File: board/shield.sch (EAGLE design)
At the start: 45 parts, among them IC1 LM75, J1 22-05-7048-04, J2 22-05-7028-02, J4 POWER_JACKPTH, K1 G5L, T1 BC817, U1 LM2596S-5.0

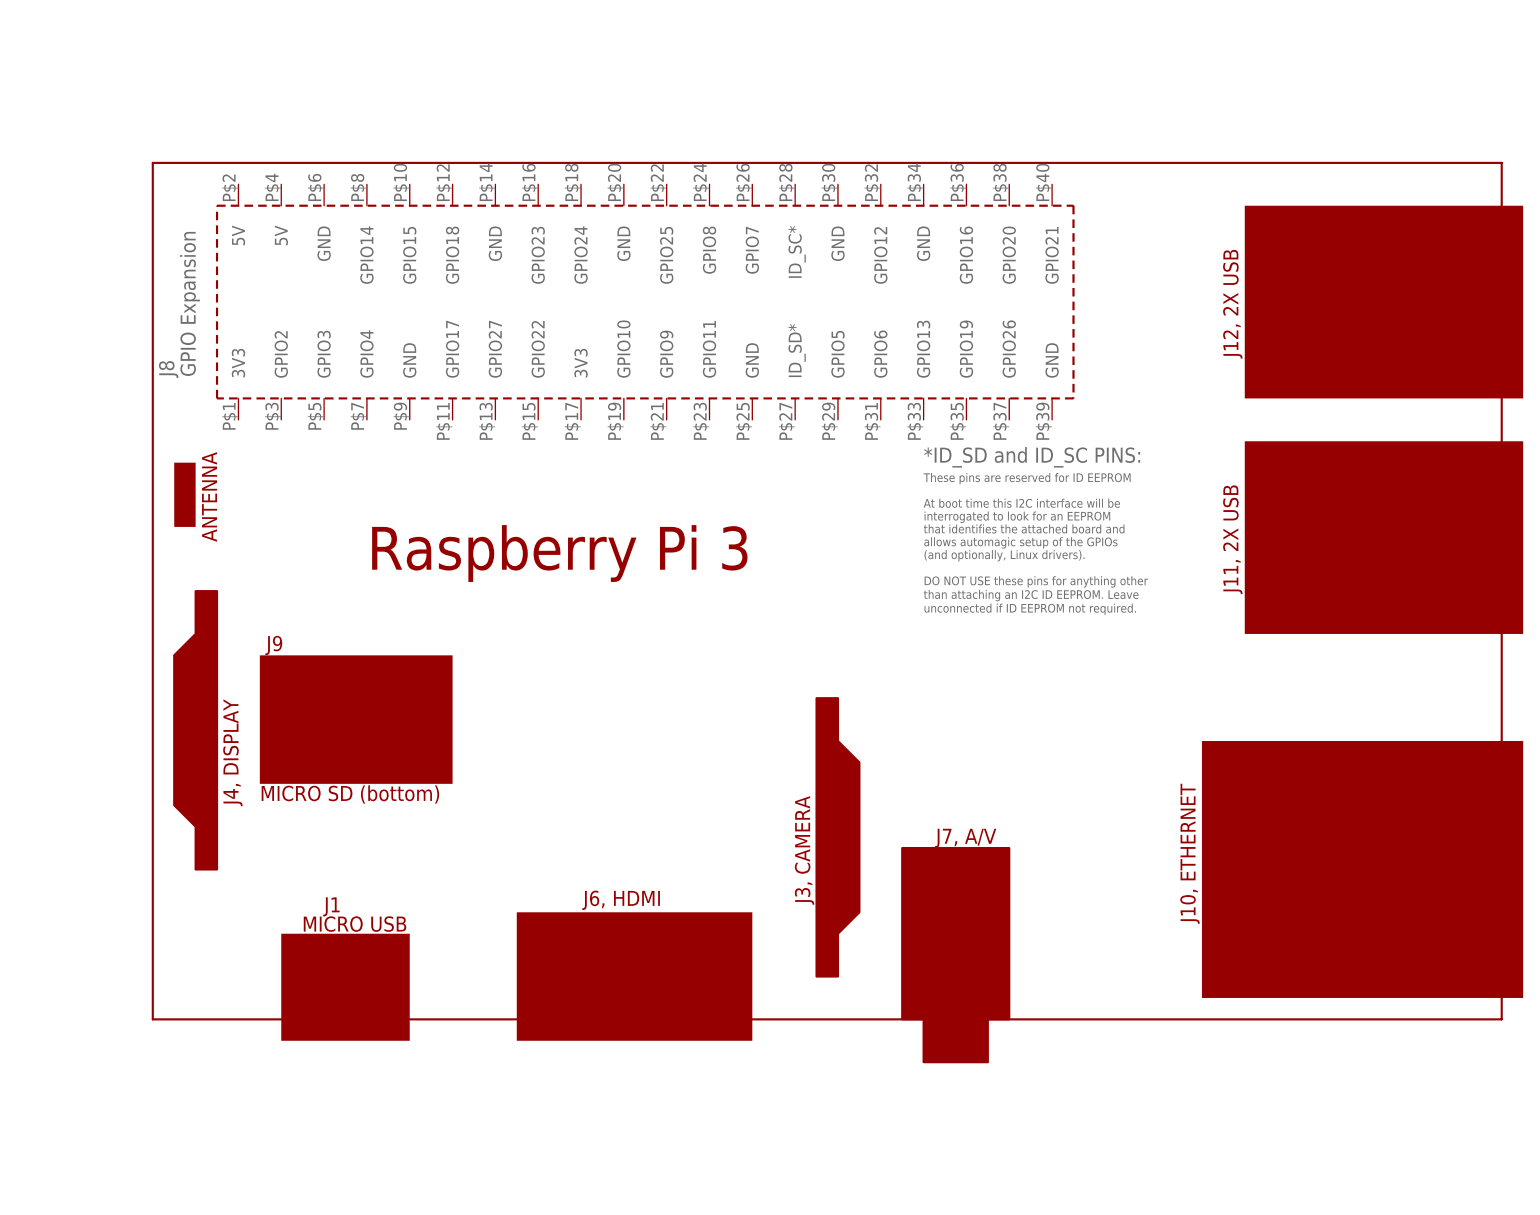
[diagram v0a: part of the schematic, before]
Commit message: Silkscreen corrected
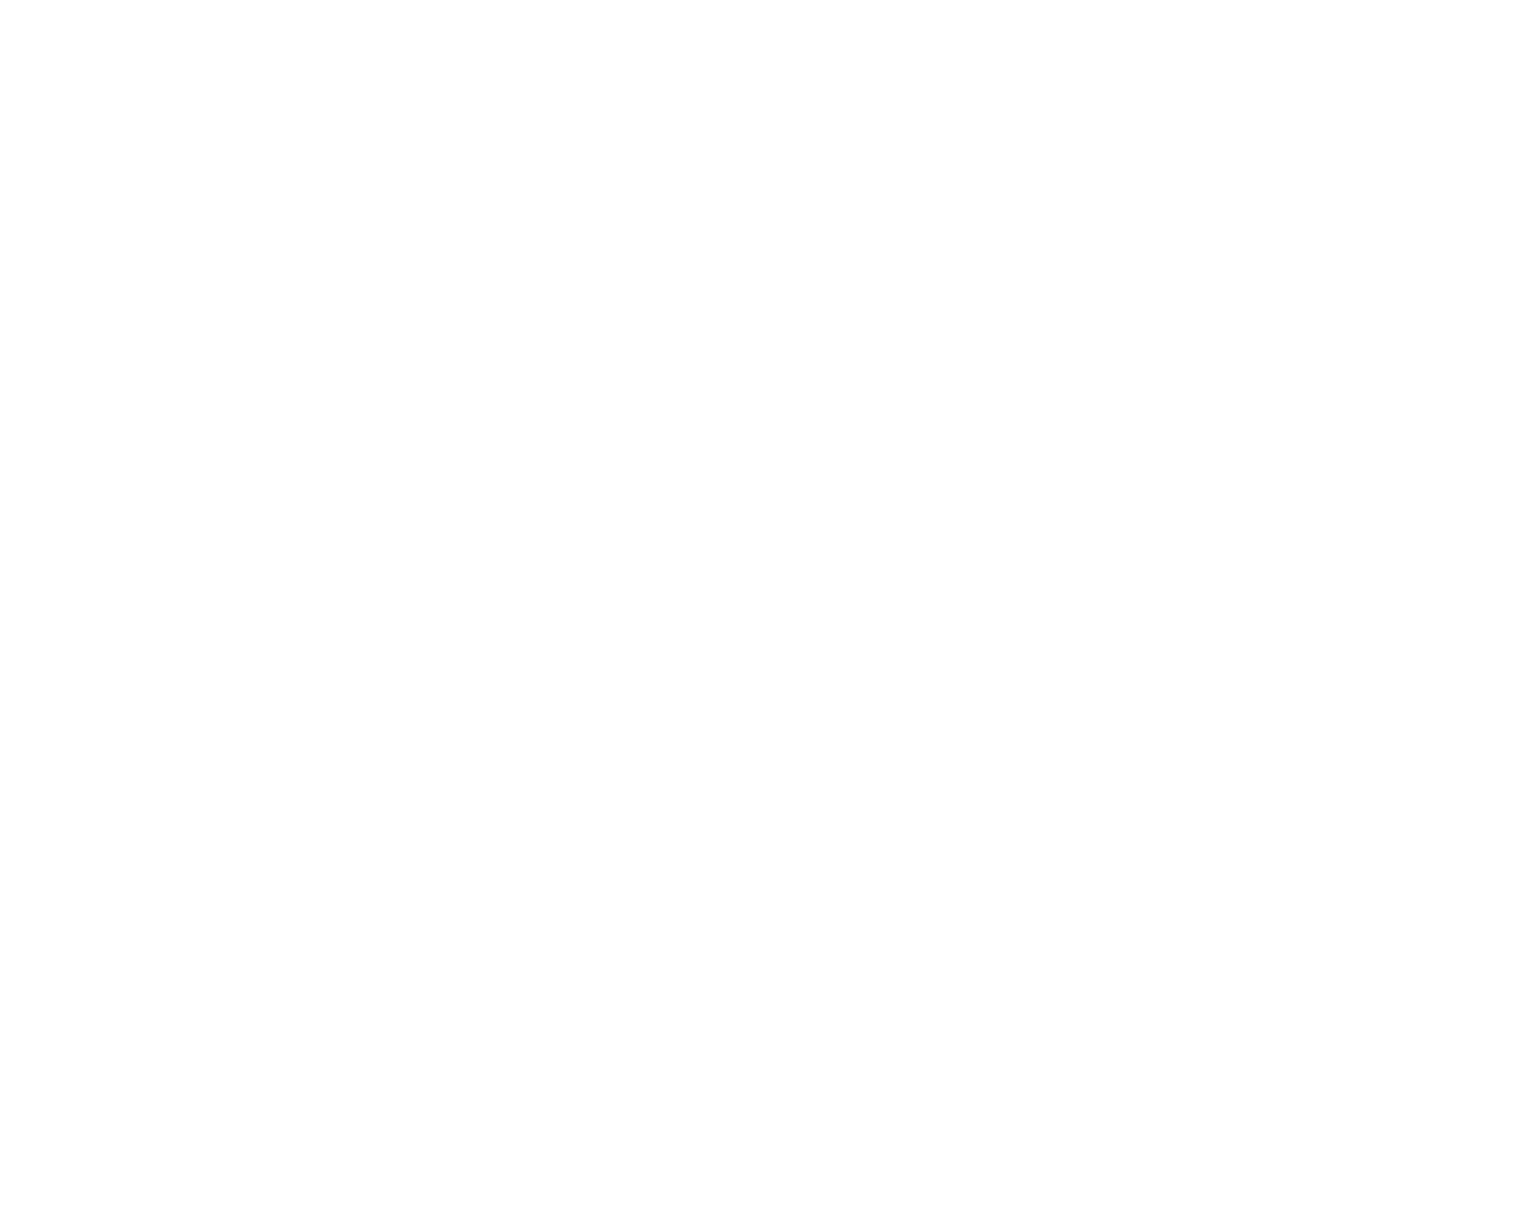
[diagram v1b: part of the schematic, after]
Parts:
- removed PCB1: RPI3, e14_Rpi3_RevA:RPI3
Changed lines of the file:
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@@
 <part name="D7" library="diode" deviceset="DIODE-" device="DO-214AC" value="1N4007 DO-214AC"/>
 <part name="F1" library="ptc-littlefuse" deviceset="1812L" device="" value="PPTC1812SMD110/16V"/>
-<part name="PCB1" library="e14_Rpi3_RevA" deviceset="RPI3" device=""/>
 <part name="P+6" library="supply1" deviceset="+5V" device=""/>
 <part name="J2" library="con-molex" deviceset="22-?-02" device="05-7028"/>
@@
 </instance>
 <instance part="F1" gate="G$1" x="175.26" y="142.24"/>
-<instance part="PCB1" gate="G$1" x="320.04" y="33.02"/>
 <instance part="P+6" gate="1" x="233.68" y="106.68" rot="MR0"/>
 <instance part="J2" gate="-1" x="180.34" y="10.16"/>
@@
 </schematic>
 </drawing>
-<compatibility>
-<note version="6.3" minversion="6.2.2" severity="warning">
-Since Version 6.2.2 text objects can contain more than one line,
-which will not be processed correctly with this version.
-</note>
-</compatibility>
 </eagle>
